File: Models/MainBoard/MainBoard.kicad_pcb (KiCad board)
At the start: 2 copper layers, 6 parts

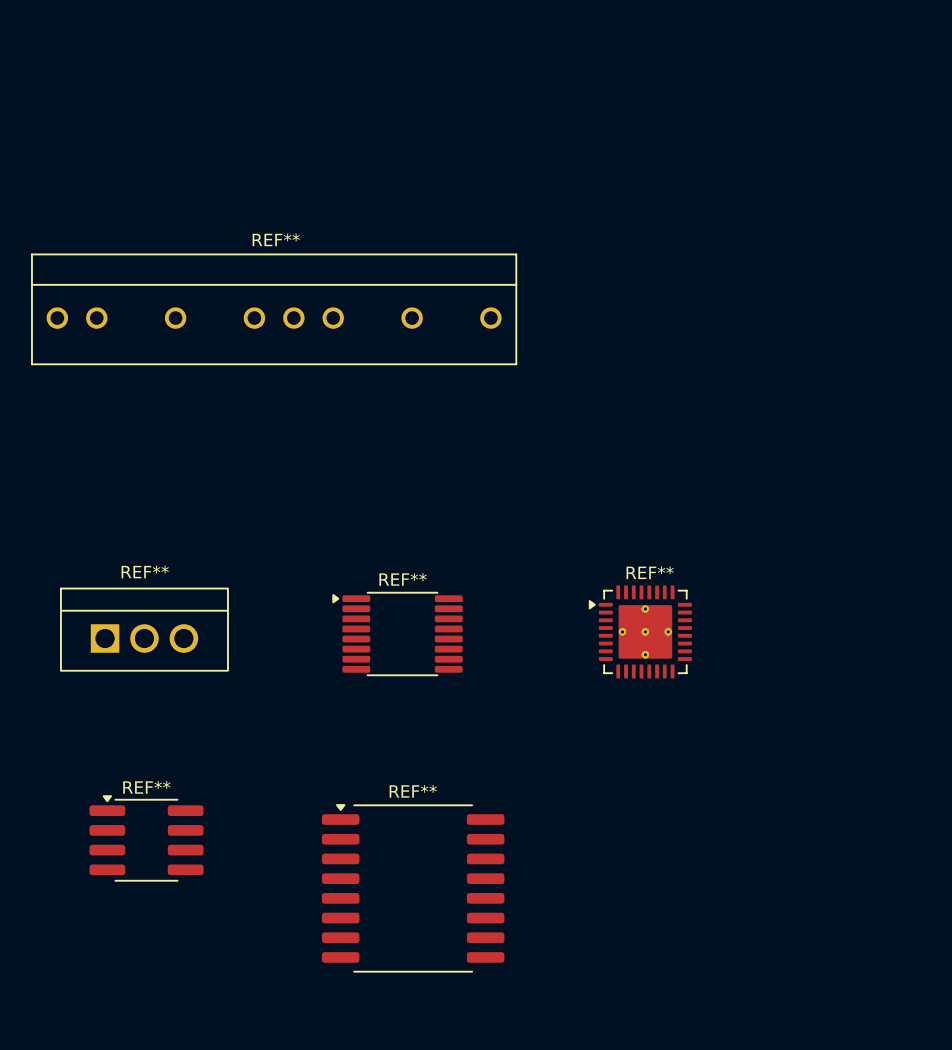
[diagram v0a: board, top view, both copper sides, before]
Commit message: Save progress
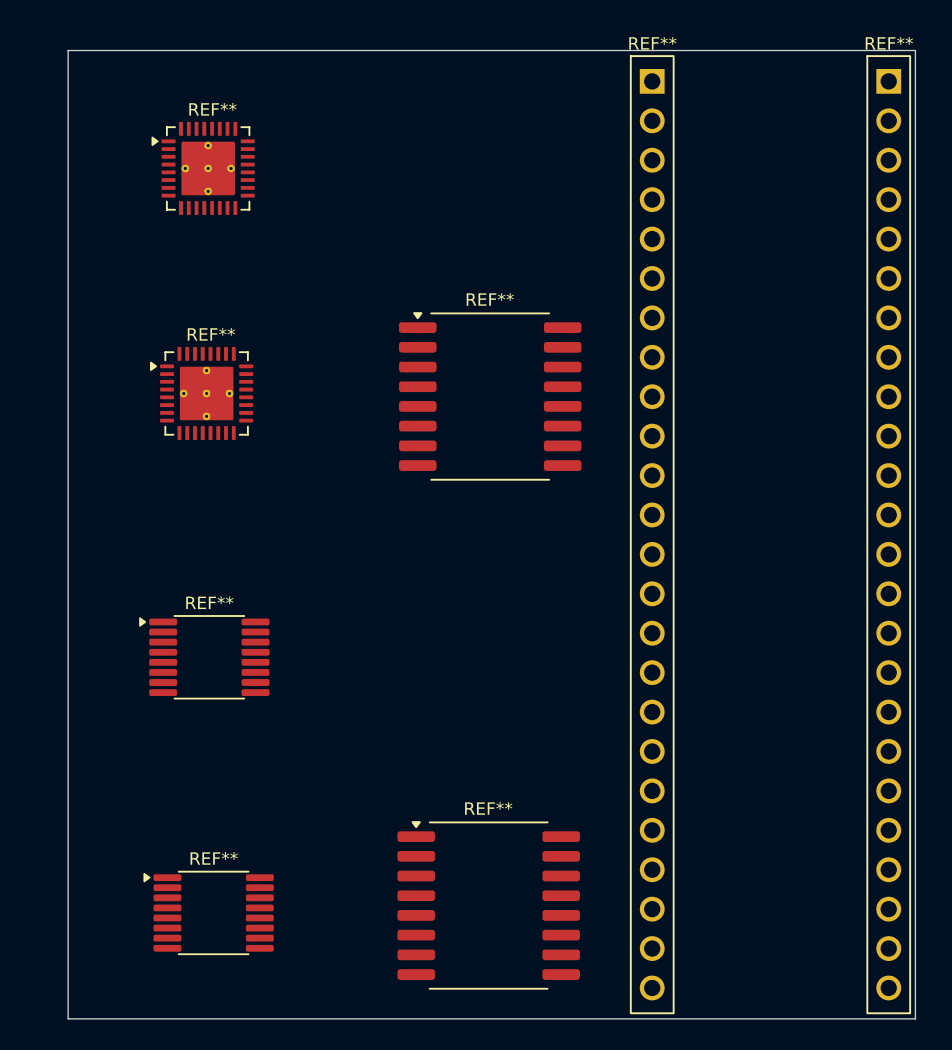
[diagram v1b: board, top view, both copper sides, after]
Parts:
- removed the REF** at (143.3, 74.9)
- removed the REF** at (151.6, 95.3)
- removed the REF** at (152.2, 111.7)
- removed the REF** at (167.2, 95.2)
- removed the REF** at (135.1, 108.6)
- removed the REF** at (134.9, 95.6)
- added REF**: TSSOP-16, IC:TSSOP-16, F.Cu at (139.1, 96.8)
- added REF**: SOIC-16-Wide, IC:SOIC-16-Wide, F.Cu at (157.1, 112.8)
- added REF**: PinSocket_1x24, Connector_Custom:PinSocket_1x24, F.Cu at (182.9, 88.9)
- added REF**: VQFN-32, IC:VQFN-32, F.Cu at (138.9, 79.8)
- added REF**: TSSOP-16, IC:TSSOP-16, F.Cu at (139.4, 113.3)
- added REF**: PinSocket_1x24, Connector_Custom:PinSocket_1x24, F.Cu at (167.6, 88.9)
- added REF**: SOIC-16-Wide, IC:SOIC-16-Wide, F.Cu at (157.2, 80.0)
- added REF**: VQFN-32, IC:VQFN-32, F.Cu at (139.0, 65.3)
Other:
- board outline added: 54.6 x 62.4 mm
- board text added: "0.1524 mm / 0.1524 mm"
- board text added: "0.2540 mm"
- board text added: "1.6256 mm"
- board text added: "2"
- board text added: "54.6000 mm x 62.4000 mm"
- board text added: "BOARD CHARACTERISTICS"
- board text added: "Board Thickness:"
- board text added: "Board overall dimensions:"
- board text added: "Castellated pads:"
- board text added: "Copper Finish:"
- board text added: "Copper Layer Count:"
- board text added: "Edge card connectors:"
- board text added: "Impedance Control:"
- board text added: "Min hole diameter:"
- board text added: "Min track/spacing:"
- board text added: "No"
- board text added: "None"
- board text added: "Plated Board Edge:"
